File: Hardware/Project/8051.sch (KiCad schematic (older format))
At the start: 0 parts

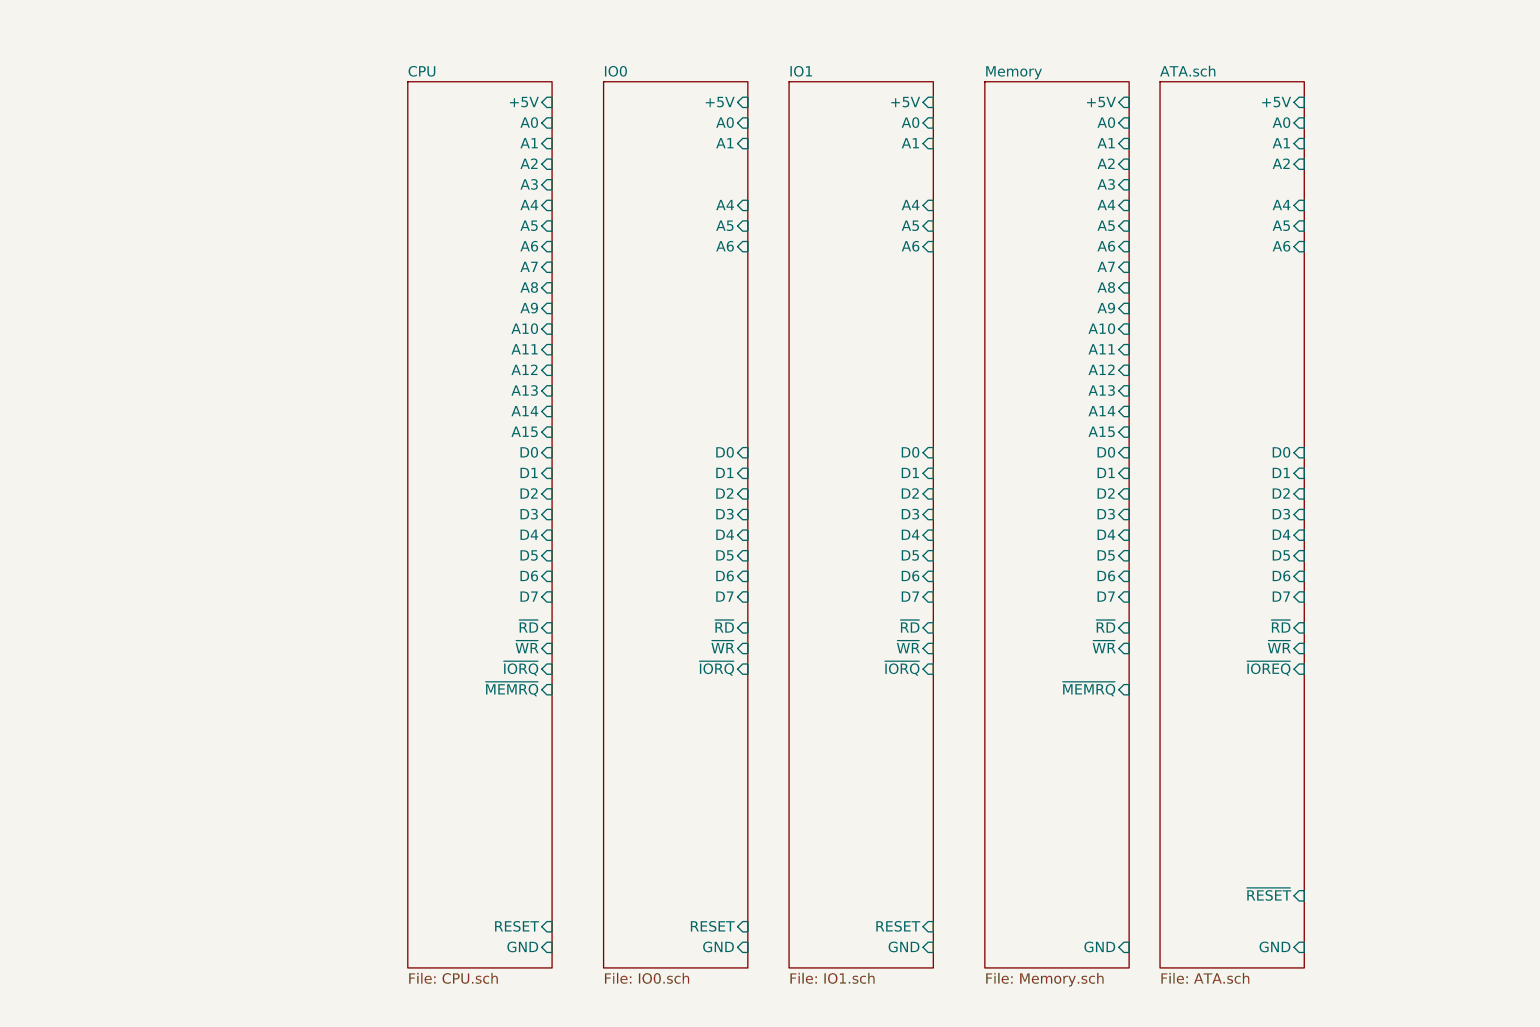
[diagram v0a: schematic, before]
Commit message: 1
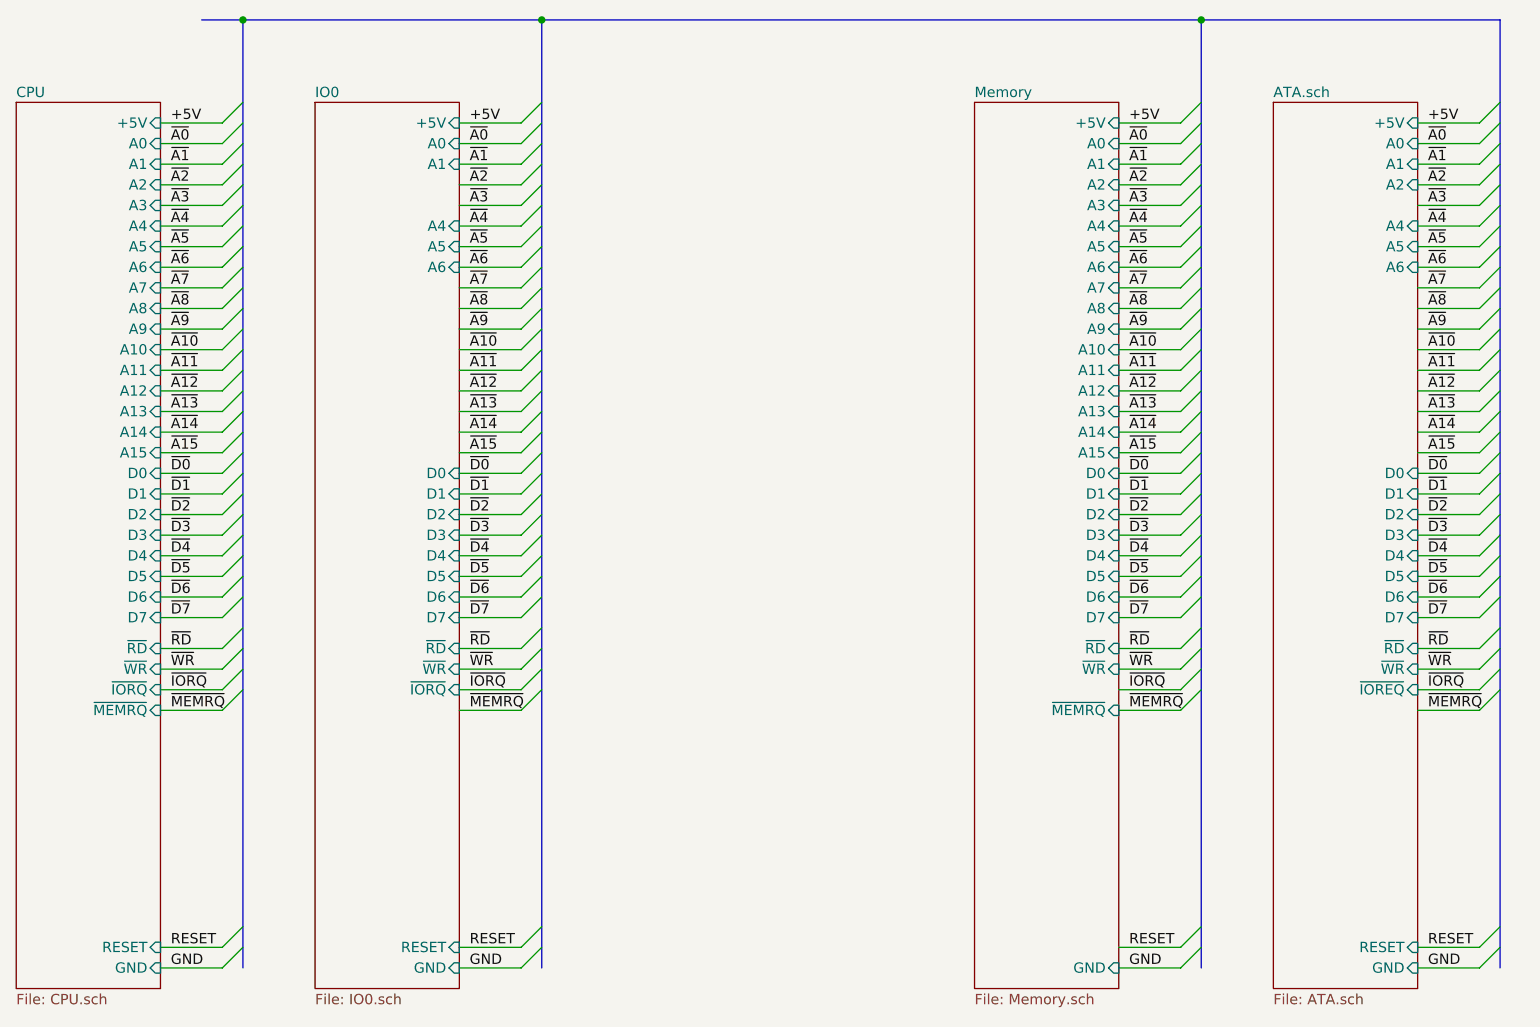
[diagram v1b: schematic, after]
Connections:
- net labels added: +5V, GND, RESET, ~A0, ~A1, ~A10, ~A11, ~A12, ~A13, ~A14, ~A15, ~A2, ~A3, ~A4, ~A5, ~A6, ~A7, ~A8, ~A9, ~D0, ~D1, ~D2, ~D3, ~D4, ~D5, ~D6, ~D7, ~IORQ, ~MEMRQ, ~RD, ~WR
- wire segments 0 -> 124
